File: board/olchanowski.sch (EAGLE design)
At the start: 164 parts, among them IC1 LPC1768, J1 B4B-XH-A(LF)(SN), J2 B4B-XH-A(LF)(SN), J3 B4B-XH-A(LF)(SN), J4 ARJM11D7-009-AB-ER2-T, J5 B4B-XH-A(LF)(SN), J6 USB-C-FEMALE, P1 TPSM53602, Q3 SIJA58DP, Q4 SIJA58DP, Q5 SSM3K329R,LF, Q6 SSM3K329R,LF, Q7 SSM3K329R,LF, Q8 SSM3K329R,LF, Q9 PFETSM, SW1 SPST-2-4PIN, SW2 SPST-2-4PIN, U1 TMC2209-LA, U2 TMC2209-LA, U3 TMC2209-LA, U4 TMC2209-LA, U5 LAN8720, U6 74HC1G04, U7 LM5111, U8 NCP5661-0, X1 X-AXIS, X2 X-AXIS, X3 X-AXIS, X4 FAN, X5 UI, X6 HB THERM

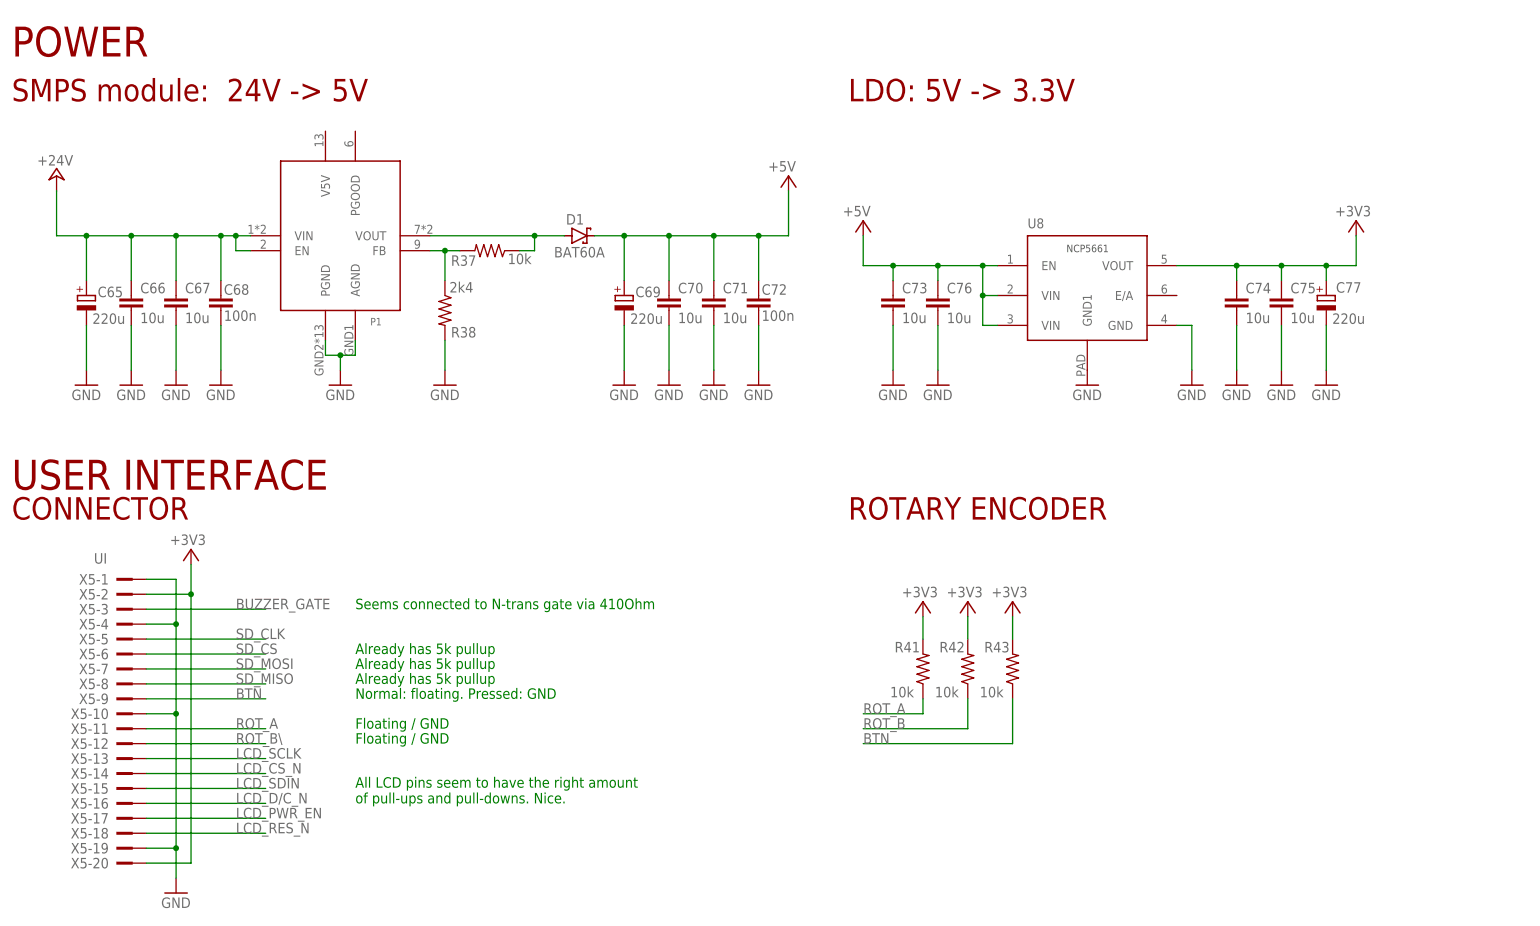
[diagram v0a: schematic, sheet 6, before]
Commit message: More stuff
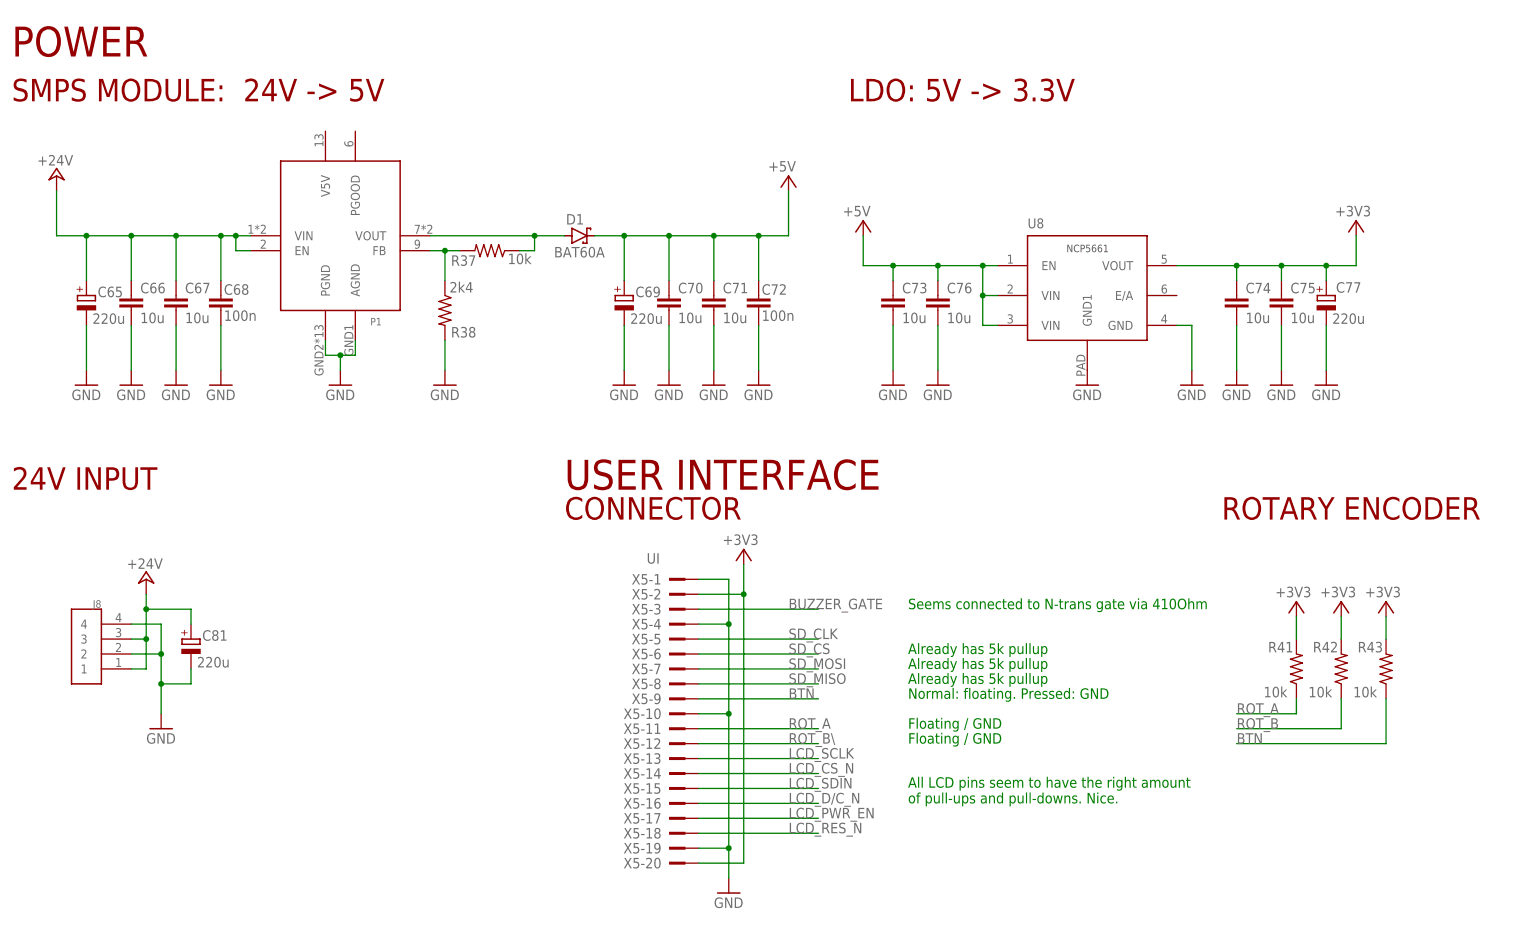
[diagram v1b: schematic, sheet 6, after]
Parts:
- added C81: (no value), rcl:CPOL-EU150CLZ-0810
- added J7: 1744428-4, robbe:1744428-4
- added J8: 282814-4, robbe:282814-4
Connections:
- new net N$61: J7.3, J7.4, Q4.D
- net +24V: now also C81.+, J7.1, J7.2, J8.1, J8.3
- net GND: now also C81.-, J8.2, J8.4
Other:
- note added: "24V INPUT"
- note added: "SMPS MODULE: 24V -> 5V"
- note removed: "SMPS module: 24V -> 5V"
- moved on the sheet: R41, R42, R43, X5-1, X5-10, X5-11, X5-12, X5-13, X5-14, X5-15, X5-16, X5-17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
